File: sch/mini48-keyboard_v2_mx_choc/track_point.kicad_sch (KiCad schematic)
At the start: 22 parts, among them J1 Conn_01x08, Q1 BSS138, Q2 BSS138, Q3 BSS138, SW100 SW_Push, SW101 SW_Push, SW102 SW_Push, SW97 SW_Push, SW98 SW_Push, SW99 SW_Push

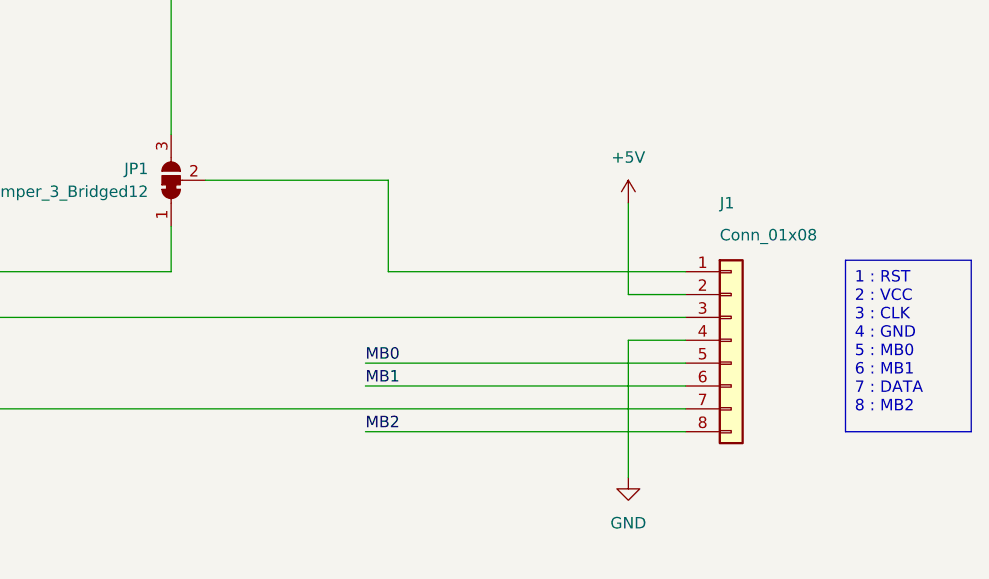
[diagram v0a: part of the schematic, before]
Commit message: KiCad のバージョンを9に上げました。
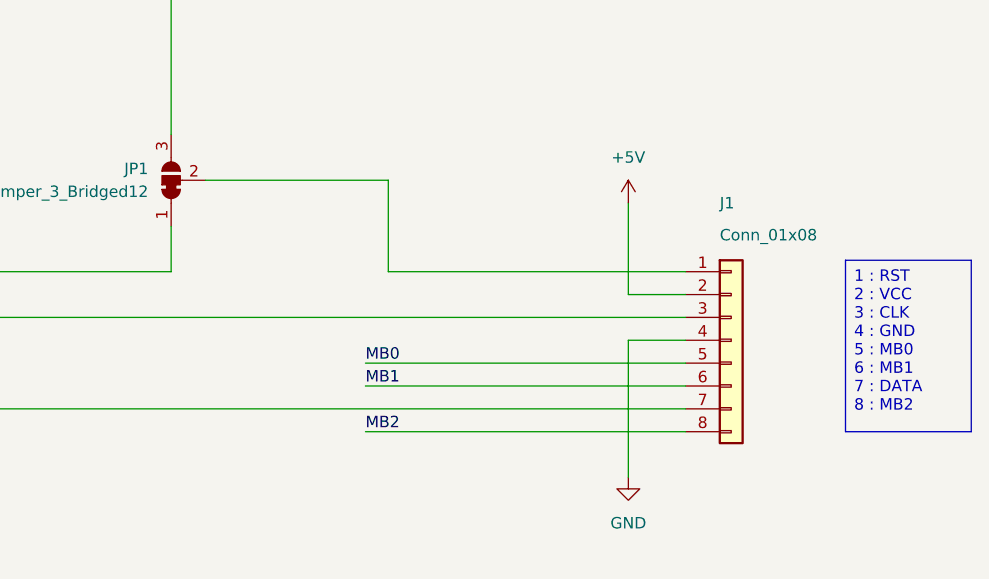
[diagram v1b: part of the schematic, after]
